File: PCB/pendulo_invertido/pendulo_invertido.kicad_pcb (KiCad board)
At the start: 2 copper layers, 106.7 x 63.5 mm, 14 parts, among them J1 Conn_01x02, J2 Conn_01x02, U1 ESP32-DevKitC V4, U2 MPU6050, U3 TB6612FNG, U5 L7805

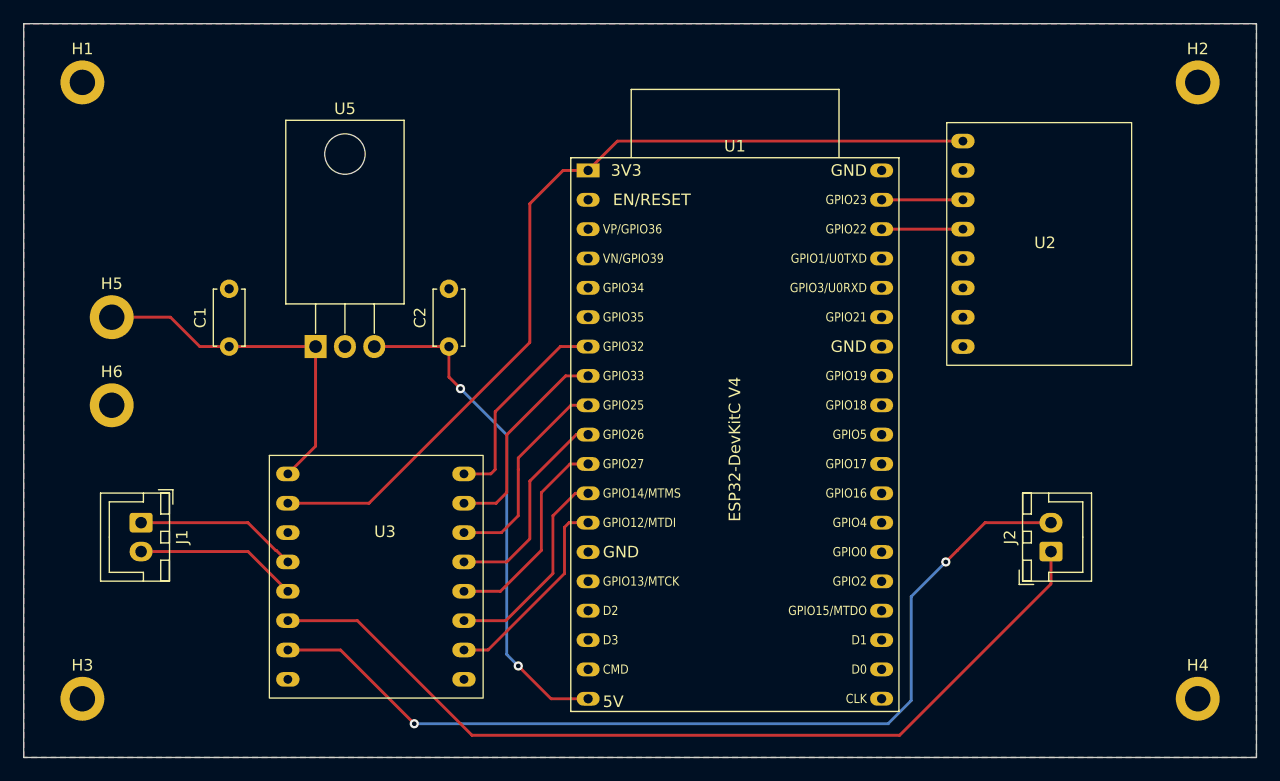
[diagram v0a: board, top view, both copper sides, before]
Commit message: modificaciones prototipo
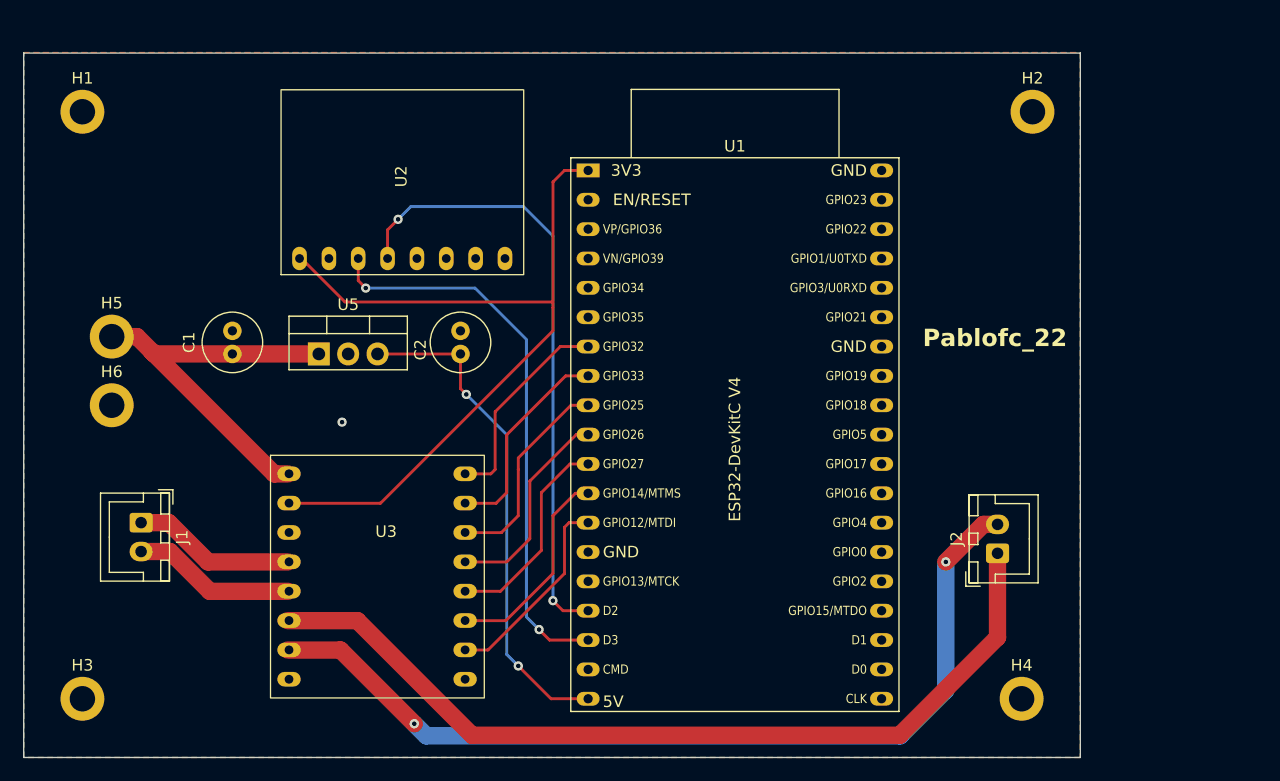
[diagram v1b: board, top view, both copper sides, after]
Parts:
- C1: value 0.1 uF -> 0.33 uF; footprint Capacitor_THT:C_Disc_D4.7mm_W2.5mm_P5.00mm -> Capacitor_THT:C_Radial_D5.0mm_H11.0mm_P2.00mm
- C2: footprint Capacitor_THT:C_Disc_D4.7mm_W2.5mm_P5.00mm -> Capacitor_THT:C_Radial_D5.0mm_H11.0mm_P2.00mm
- U5: footprint Package_TO_SOT_THT:TO-220-3_Horizontal_TabDown -> Package_TO_SOT_THT:TO-220-3_Vertical
- moved U2 58.3 mm to (100.1, 78.7), turned to 90 degrees
- moved H4 15.2 mm to (162.6, 116.8)
- moved H2 14.5 mm to (163.5, 66.0)
- moved J2 4.63 mm to (160.5, 104.2)
- moved H1 2.54 mm to (81.3, 66.0)
- moved H5 1.68 mm to (83.8, 85.5)
- moved C2 1.19 mm to (114.0, 87.0)
- moved C1 0.70 mm to (94.3, 87.0)
- moved U5 0.70 mm to (101.7, 87.0)
- moved U3 0.10 mm to (99.2, 97.4)
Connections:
- U1 pad 16: unconnected-(U1-D2-Pad16) -> Net-(U1-D2)
- U1 pad 17: unconnected-(U1-D3-Pad17) -> Net-(U1-D3)
- U1 pad 36: Net-(U1-22) -> unconnected-(U1-22-Pad36)
- U1 pad 37: Net-(U1-23) -> unconnected-(U1-23-Pad37)
- U2 pad 3: Net-(U1-23) -> Net-(U1-D3)
- U2 pad 4: Net-(U1-22) -> Net-(U1-D2)
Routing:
- net Net-(U1-D2): track 0.00 -> 53.6 mm, vias 0 -> 2
- net Net-(U1-D3): track 0.00 -> 48.7 mm, vias 0 -> 2
- net Net-(U1-3V3): track 78.4 -> 69.0 mm
- net Net-(U1-23): track 7.04 -> 0.00 mm
- net Net-(U1-22): track 7.04 -> 0.00 mm
- net +6V: track 30.7 -> 34.8 mm
- net Net-(J2-Pin_2): track 81.2 -> 78.6 mm
- net Net-(J2-Pin_1): track 78.4 -> 76.3 mm
- net Net-(U1-5V): track 43.8 -> 43.1 mm
- net GND: vias 0 -> 1
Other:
- board size 106.7 x 63.5 mm -> 91.4 x 61 mm
- board text added: "Pablofc_22"
